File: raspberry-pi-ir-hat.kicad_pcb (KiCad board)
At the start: 2 copper layers, 40.3 x 85 mm, 20 parts, among them J1 IO, J2 TX, J3 RX, J4 RX_JMP, J5 TX_JMP, J6 RW_JMP, J7 Raspberry_Pi_2_3, Q1 Q_NMOS_GSD

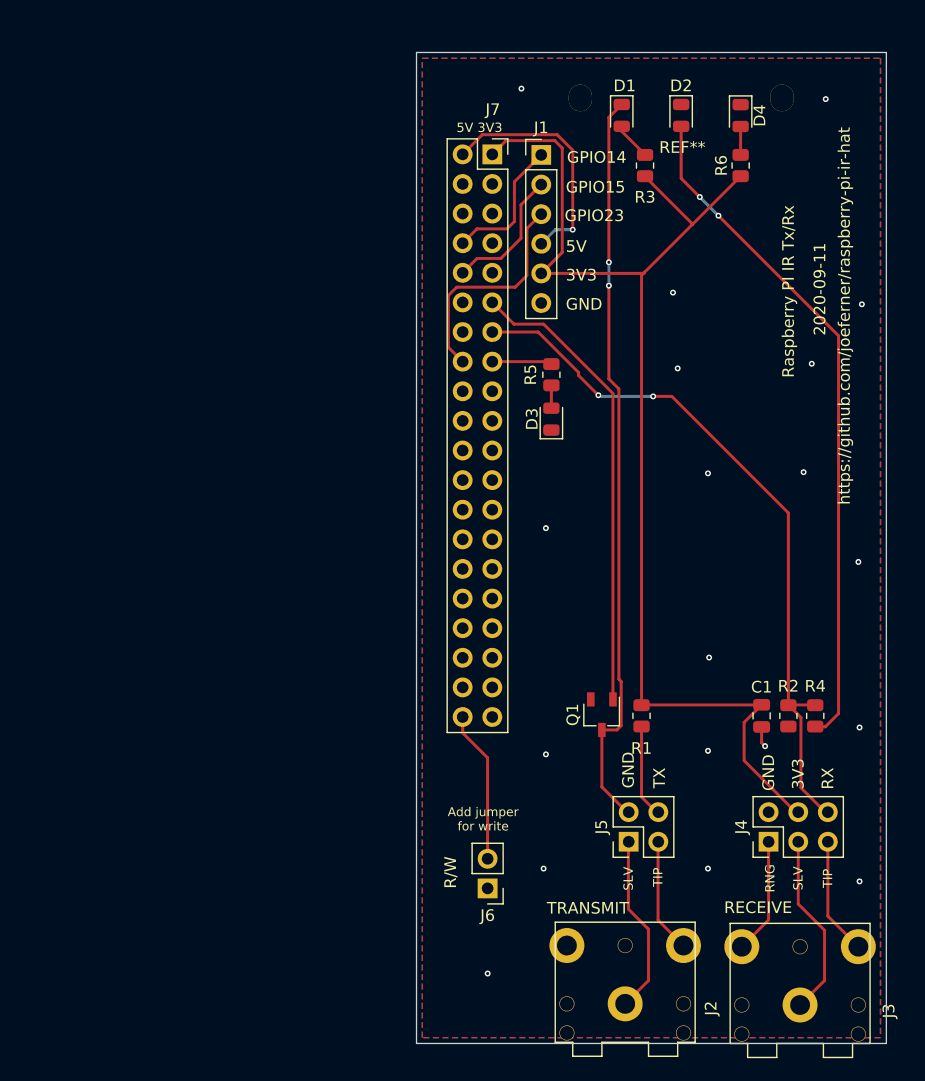
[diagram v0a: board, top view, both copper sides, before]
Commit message: 2020-10-01
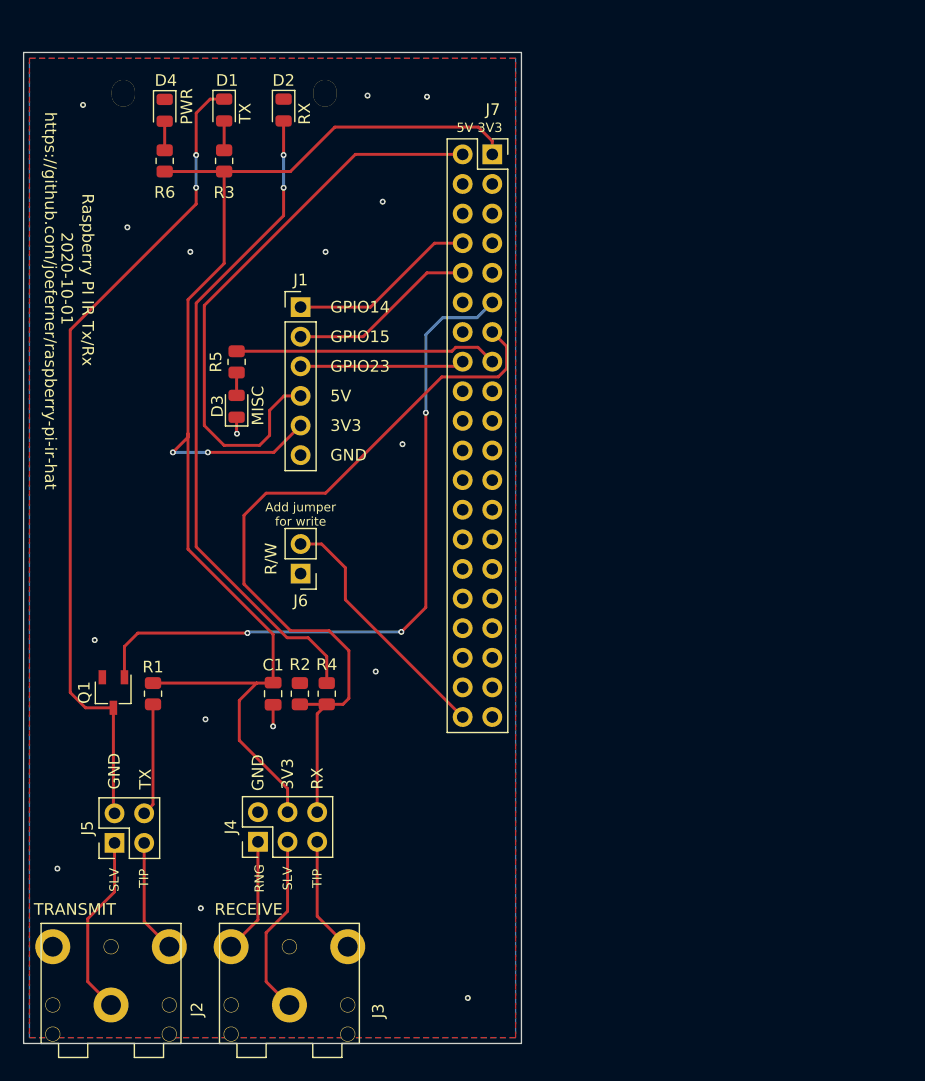
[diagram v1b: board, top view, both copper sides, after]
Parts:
- moved D4 49.4 mm to (118.1, 81.0)
- moved R6 49.4 mm to (118.1, 85.3)
- moved J5 44.1 mm to (113.8, 143.8)
- moved J2 44.1 mm to (113.5, 157.7)
- moved J4 43.8 mm to (126.1, 143.7)
- moved J3 43.8 mm to (128.8, 157.7)
- moved C1 41.9 mm to (127.4, 131.0)
- moved R1 41.9 mm to (117.1, 131.0)
- moved R2 41.9 mm to (129.7, 131.0), turned to 90 degrees
- moved R4 41.9 mm to (132.0, 131.0), turned to 90 degrees
- moved Q1 41.9 mm to (113.7, 130.9)
- moved REF** 39.2 mm to (123.2, 80.8)
- moved R3 36.1 mm to (123.2, 85.3)
- moved D1 34.1 mm to (123.2, 80.9)
- moved D2 34.1 mm to (128.3, 80.9)
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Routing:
- net /5V: track 20.7 -> 49.8 mm, vias 1 -> 0
- net /TX: track 39.8 -> 60.1 mm, vias 0 -> 3
- net /MISC: track 5.15 -> 22.6 mm
- net VCC: track 104.1 -> 117.2 mm, vias 0 -> 2
- net /RW: track 13.0 -> 21.7 mm
- net Net-(D1-Pad1): track 64.1 -> 70.4 mm
- net /IO3: track 19.4 -> 14.1 mm
- net /RX: track 61.6 -> 66.8 mm, vias 2 -> 0
- net /IO2: track 11.6 -> 16.2 mm
- net /IO1: track 11.9 -> 16.2 mm
- net Net-(J5-Pad4): track 8.03 -> 9.66 mm
- net GND: track 1.77 -> 3.27 mm, vias 19 -> 16
- net Net-(D2-Pad2): track 58.4 -> 57.0 mm
- net Net-(D1-Pad2): track 3.25 -> 2.51 mm
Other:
- board size 40.3 x 85 mm -> 42.7 x 85 mm
- rule solder_mask_min_width: 0.1016 -> 0.127
- board text added: "2020-10-01"
- board text added: "MISC"
- board text added: "PWR"
- board text removed: "2020-09-11"
